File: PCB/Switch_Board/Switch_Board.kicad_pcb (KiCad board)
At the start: 2 copper layers, 91.8 x 33.8 mm, 9 parts

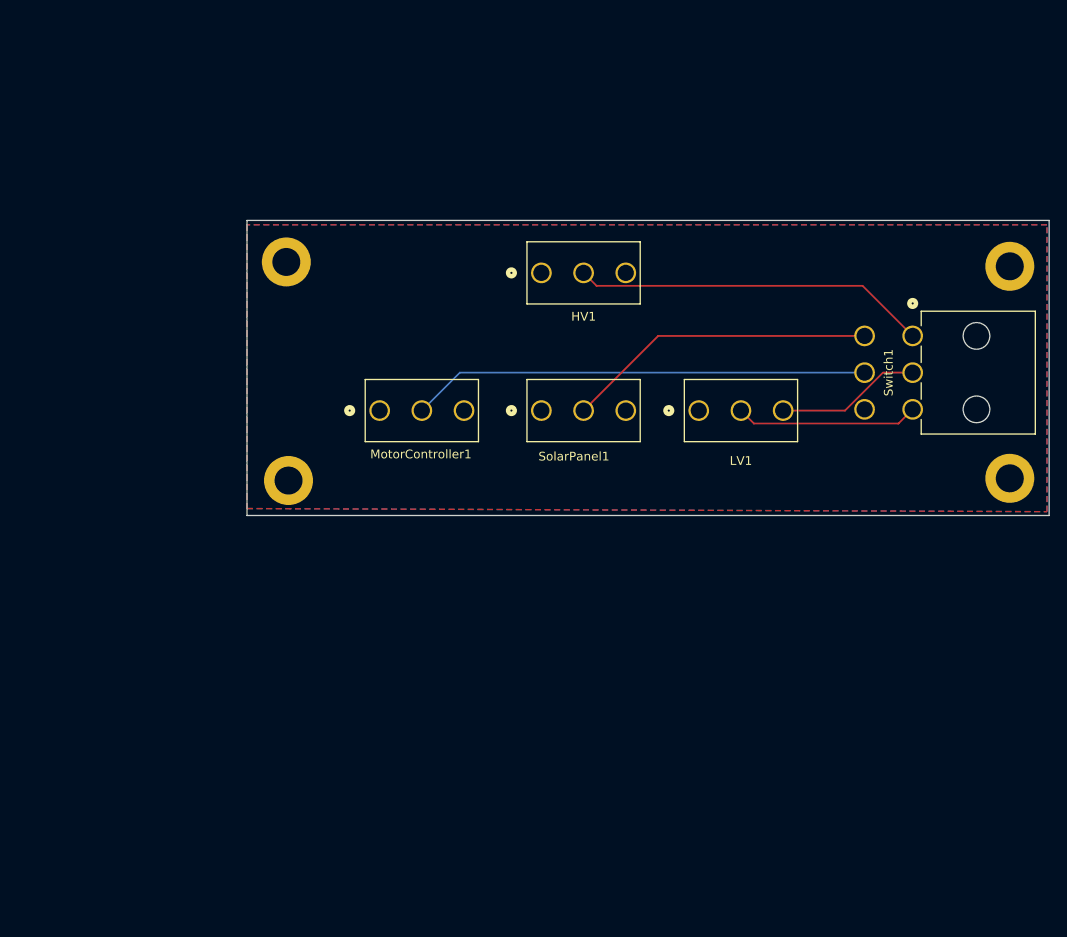
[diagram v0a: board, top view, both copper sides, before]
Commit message: Updated Version_04_13
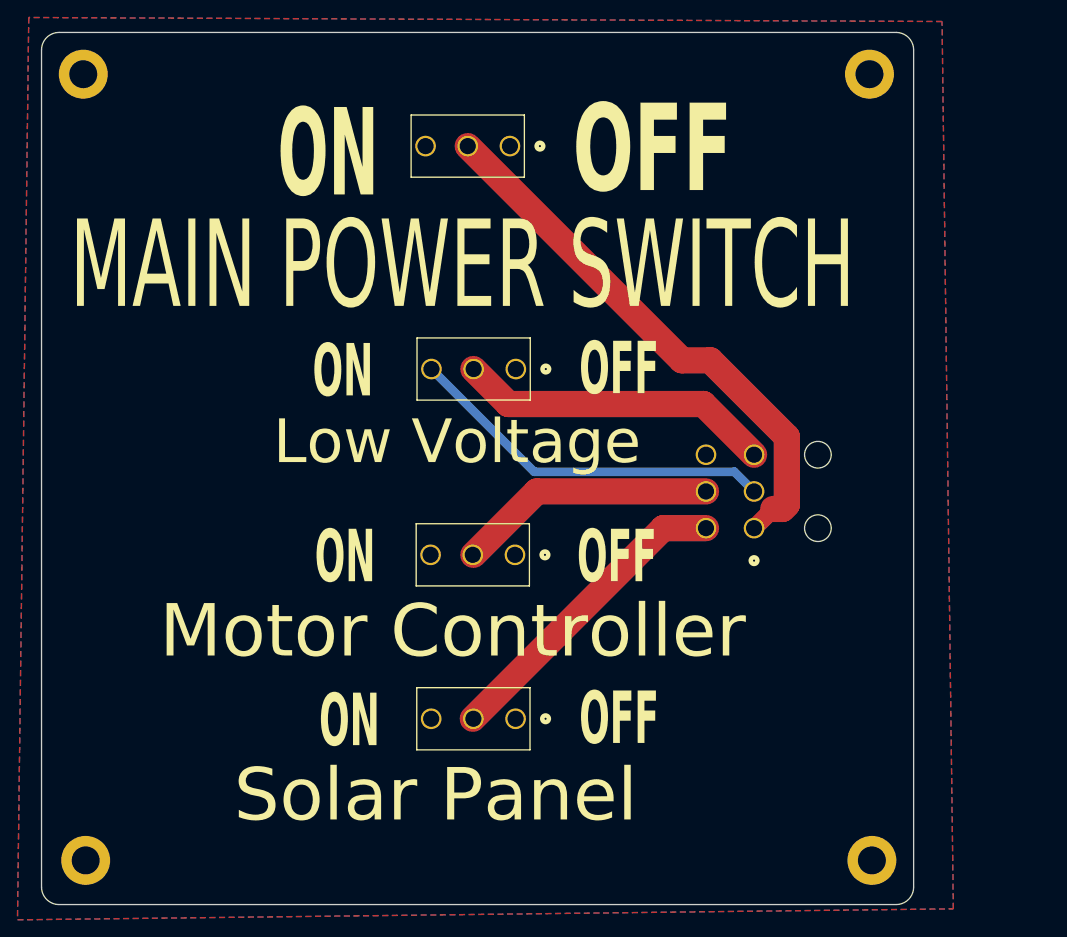
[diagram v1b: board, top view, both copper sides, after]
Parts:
- Main Power Switch: renamed from HV1
- Switch1: moved to B.Cu
- moved REF** 49.3 mm to (72.3, 132.2)
- moved REF** 46.5 mm to (162.2, 132.2)
- moved SolarPanel 35.4 mm to (121.5, 116.0), turned to 180 degrees
- moved REF** 31.6 mm to (72.0, 42.3)
- moved Switch1 28.5 mm to (148.8, 94.2), turned to -90 degrees
- moved REF** 27.2 mm to (161.9, 42.3)
- moved MotorController 22.6 mm to (121.4, 97.2), turned to 180 degrees
- moved LowVoltage 21.5 mm to (121.5, 76.0), turned to 180 degrees
- moved Main Power Switch 14.9 mm to (120.8, 50.5), turned to 180 degrees
- renumbered LV1 to LowVoltage, MotorController1 to MotorController, SolarPanel1 to SolarPanel
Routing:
- net Net-(LV1-A): track 16.6 -> 42.7 mm
- net Net-(MotorController1-B): track 52.4 -> 29.6 mm
- net Net-(HV1-B): track 40.6 -> 62.9 mm
- net Net-(LV1-B): track 20.9 -> 36.2 mm
- net unconnected-(LV1-C-Pad1): track 0.00 -> 0.71 mm
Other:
- board size 91.8 x 33.8 mm -> 99.8 x 99.8 mm
- board text added: "Low Voltage"
- board text added: "MAIN POWER SWITCH"
- board text added: "Motor Controller"
- board text added: "OFF"
- board text added: "ON"
- board text added: "Solar Panel"
